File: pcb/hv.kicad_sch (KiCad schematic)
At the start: 28 parts, among them Q1 DMN3404L

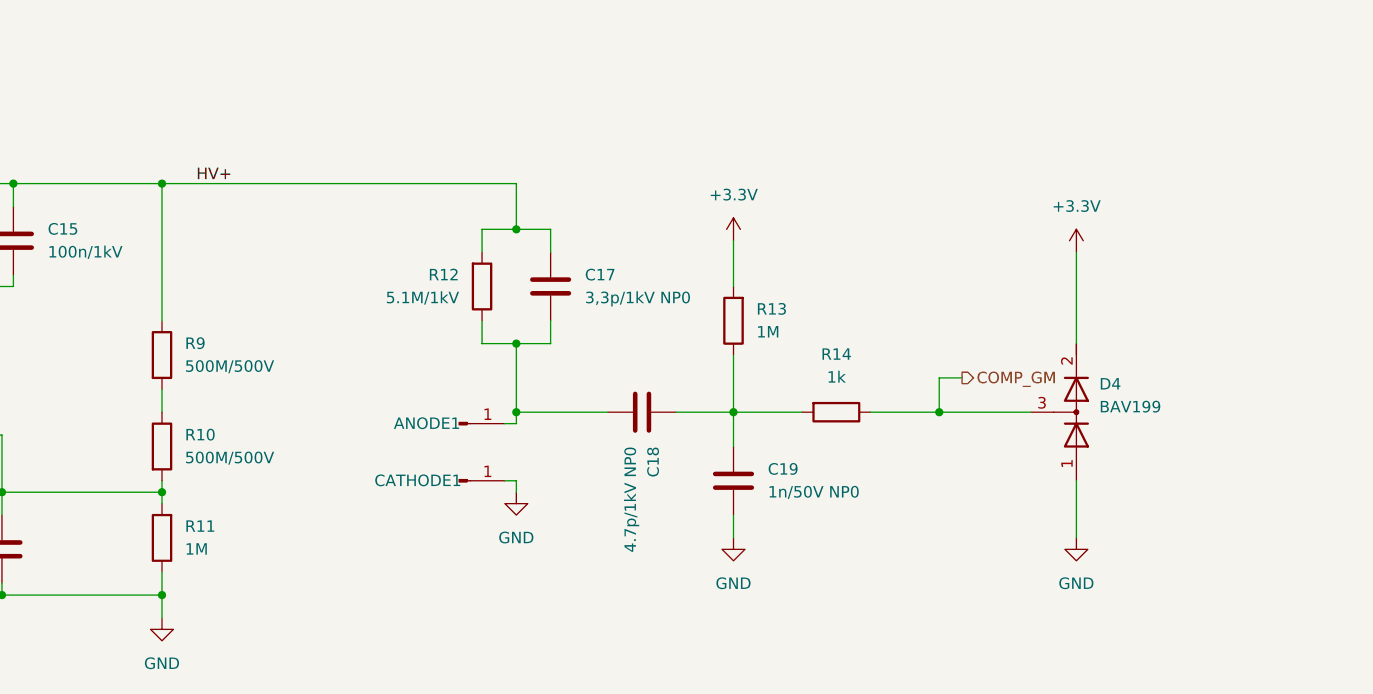
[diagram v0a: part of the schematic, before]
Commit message: Schematic finished, first routing
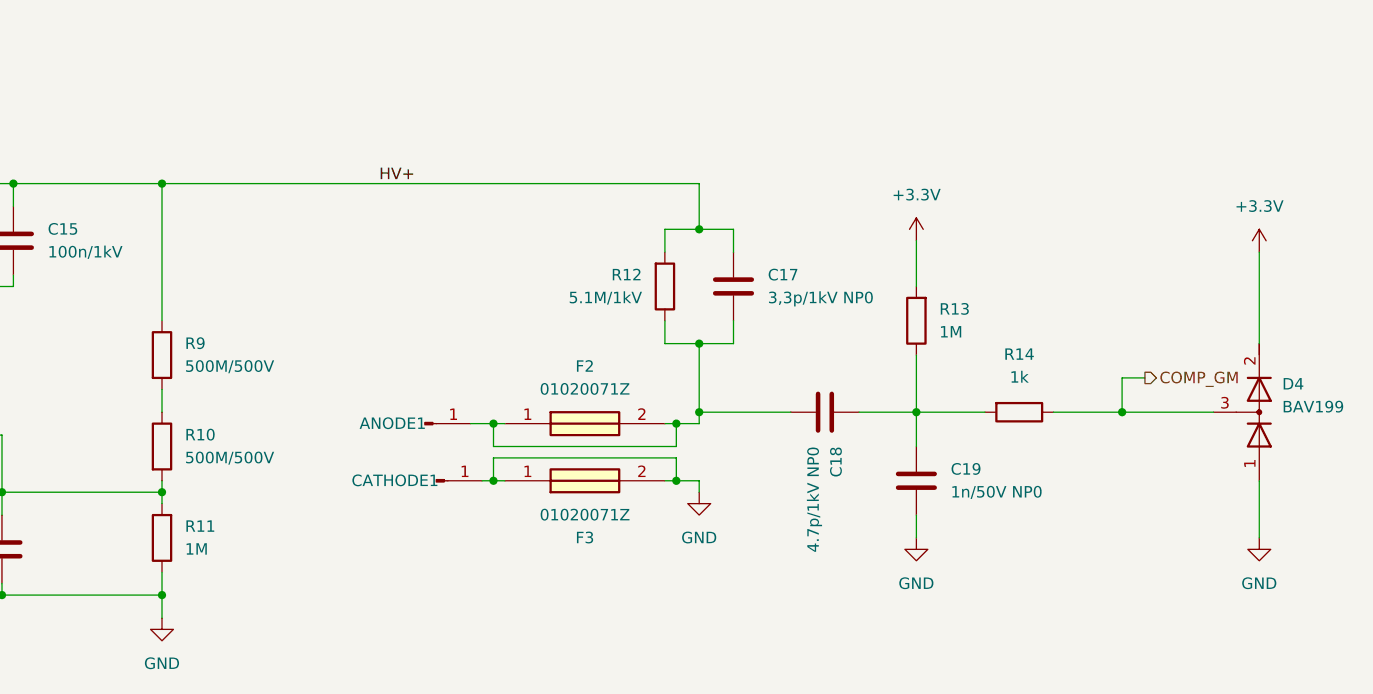
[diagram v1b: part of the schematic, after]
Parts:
- added F2, F3: 01020071Z, 01020071Z, symbol SamacSys_Parts:01020071Z
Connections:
- net GND: now also F3.1, F3.2
- net at ANODE1.1 (Pin_1), C17.2, C18.2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: now also F2.1, F2.2
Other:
- moved on the sheet: ANODE1, C17, C18, C19, CATHODE1, D4, R12, R13, R14
